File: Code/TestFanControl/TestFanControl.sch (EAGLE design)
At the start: 6 parts, among them T1 BC548

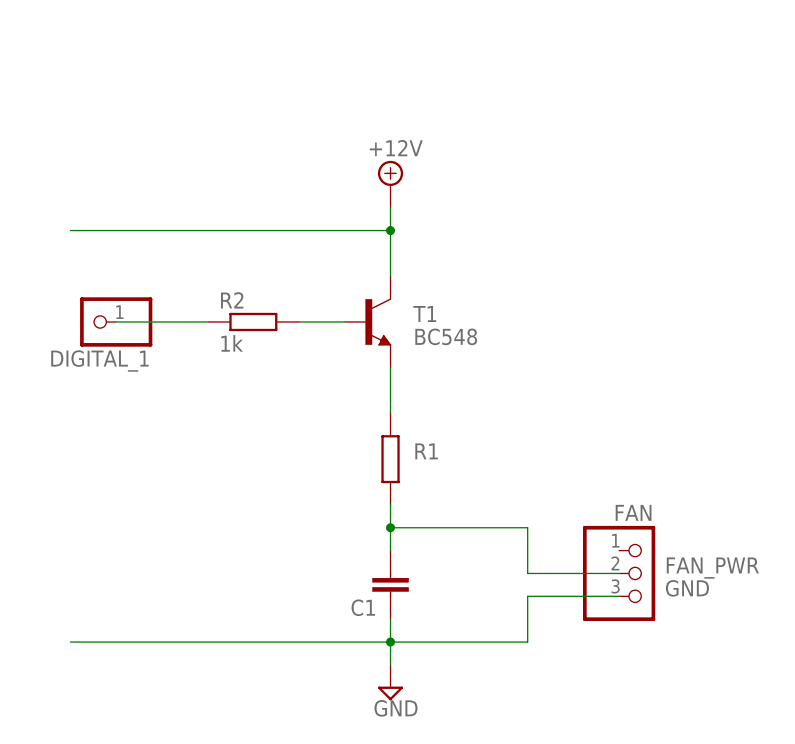
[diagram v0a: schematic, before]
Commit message: Testing
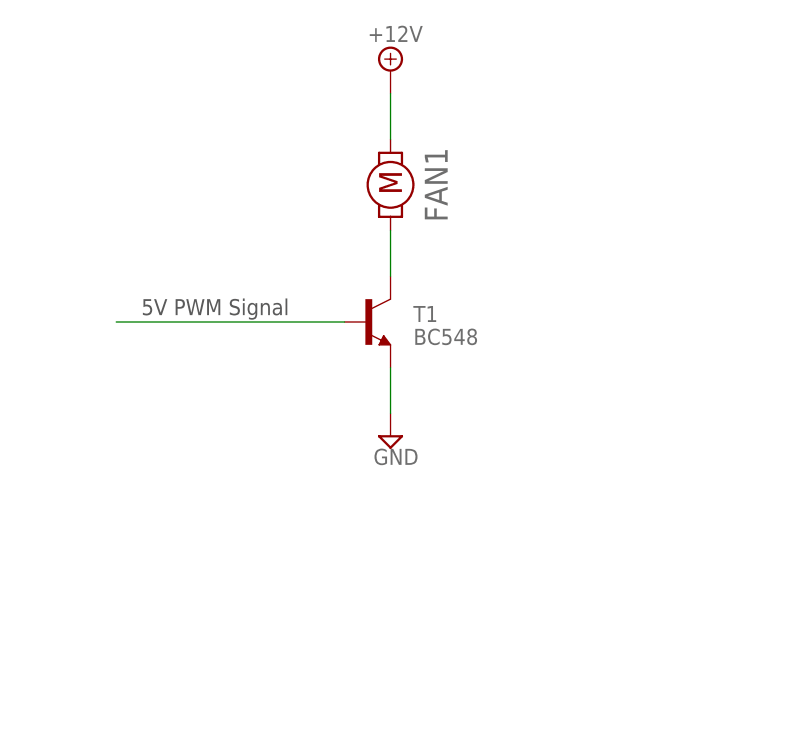
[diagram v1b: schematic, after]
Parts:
- removed C1: (no value), rcl:C-EU025-024X044
- removed DIGITAL_1: (no value), pinhead:PINHD-1X1
- removed FAN: (no value), pinhead:PINHD-1X3
- removed R1: (no value), rcl:R-EU_0204/7
- removed R2: 1k, rcl:R-EU_0204/7
- added FAN1: FAN, EnigmaMon:FAN
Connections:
- removed net FAN7_PWM: DIGITAL_1.1, R2.1
- removed net FAN_PWR: C1.2, FAN.2, R1.2
- removed net N$9: R1.1, T1.E
- new net N$2: FAN1.1, T1.C
- net +12V: now also FAN1.2; no longer T1.C
- net GND: now also T1.E; no longer C1.1, FAN.3
- net N$8: no longer R2.2
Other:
- note added: "5V PWM Signal"
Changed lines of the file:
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@@
 </classes>
 <parts>
-<part name="FAN" library="pinhead" deviceset="PINHD-1X3" device=""/>
 <part name="SUPPLY13" library="EnigmaMon" deviceset="+12V" device=""/>
 <part name="SUPPLY2" library="Rodentometer" deviceset="GND" device=""/>
 <part name="T1" library="transistor" deviceset="BC547" device="" value="BC548"/>
-<part name="R2" library="rcl" deviceset="R-EU_" device="0204/7" value="1k"/>
-<part name="DIGITAL_1" library="pinhead" deviceset="PINHD-1X1" device=""/>
-<part name="R1" library="rcl" deviceset="R-EU_" device="0204/7"/>
-<part name="C1" library="rcl" deviceset="C-EU" device="025-024X044"/>
+<part name="FAN1" library="EnigmaMon" deviceset="FAN" device=""/>
 </parts>
 <sheets>
 <sheet>
 <plain>
+<text x="5.334" y="49.022" size="1.778" layer="97">5V PWM Signal</text>
 </plain>
 <instances>
-<instance part="FAN" gate="A" x="60.96" y="20.32" smashed="yes">
-<attribute name="VALUE" x="59.69" y="12.7" size="1.778" layer="96"/>
-<attribute name="NAME" x="62.23" y="26.162" size="1.778" layer="95" rot="MR0"/>
-</instance>
-<instance part="SUPPLY13" gate="+12V" x="33.02" y="63.5"/>
-<instance part="SUPPLY2" gate="GND" x="33.02" y="7.62"/>
+<instance part="SUPPLY13" gate="+12V" x="33.02" y="76.2"/>
+<instance part="SUPPLY2" gate="GND" x="33.02" y="35.56"/>
 <instance part="T1" gate="G$1" x="30.48" y="48.26" smashed="yes">
 <attribute name="NAME" x="35.56" y="48.26" size="1.778" layer="95"/>
 <attribute name="VALUE" x="35.56" y="45.72" size="1.778" layer="96"/>
 </instance>
-<instance part="R2" gate="G$1" x="17.78" y="48.26"/>
-<instance part="DIGITAL_1" gate="G$1" x="0" y="48.26" rot="R180"/>
-<instance part="R1" gate="G$1" x="33.02" y="33.02" smashed="yes" rot="R270">
-<attribute name="NAME" x="35.56" y="32.9946" size="1.778" layer="95"/>
-<attribute name="VALUE" x="35.56" y="33.02" size="1.778" layer="96"/>
-</instance>
-<instance part="C1" gate="G$1" x="33.02" y="17.78" rot="R180"/>
+<instance part="FAN1" gate="G$1" x="33.02" y="63.5" rot="R90"/>
 </instances>
 <busses>
@@
 <segment>
 <pinref part="SUPPLY13" gate="+12V" pin="+12V"/>
-<pinref part="T1" gate="G$1" pin="C"/>
-<wire x1="33.02" y1="60.96" x2="33.02" y2="58.42" width="0.1524" layer="91"/>
-<wire x1="33.02" y1="58.42" x2="33.02" y2="53.34" width="0.1524" layer="91"/>
-<wire x1="33.02" y1="58.42" x2="-2.54" y2="58.42" width="0.1524" layer="91"/>
-<junction x="33.02" y="58.42"/>
-</segment>
-</net>
-<net name="GND" class="0">
-<segment>
-<wire x1="33.02" y1="15.24" x2="33.02" y2="12.7" width="0.1524" layer="91"/>
-<pinref part="SUPPLY2" gate="GND" pin="GND"/>
-<pinref part="C1" gate="G$1" pin="1"/>
-<pinref part="FAN" gate="A" pin="3"/>
-<wire x1="33.02" y1="12.7" x2="33.02" y2="10.16" width="0.1524" layer="91"/>
-<wire x1="58.42" y1="17.78" x2="48.26" y2="17.78" width="0.1524" layer="91"/>
-<wire x1="48.26" y1="17.78" x2="48.26" y2="12.7" width="0.1524" layer="91"/>
-<wire x1="48.26" y1="12.7" x2="33.02" y2="12.7" width="0.1524" layer="91"/>
-<label x="63.5" y="17.78" size="1.778" layer="95"/>
-<junction x="33.02" y="12.7"/>
-<wire x1="33.02" y1="12.7" x2="-2.54" y2="12.7" width="0.1524" layer="91"/>
+<wire x1="33.02" y1="68.58" x2="33.02" y2="73.66" width="0.1524" layer="91"/>
+<pinref part="FAN1" gate="G$1" pin="2"/>
 </segment>
 </net>
@@
 <segment>
 <pinref part="T1" gate="G$1" pin="B"/>
-<wire x1="27.94" y1="48.26" x2="22.86" y2="48.26" width="0.1524" layer="91"/>
-<pinref part="R2" gate="G$1" pin="2"/>
+<wire x1="27.94" y1="48.26" x2="2.54" y2="48.26" width="0.1524" layer="91"/>
 </segment>
 </net>
-<net name="FAN7_PWM" class="0">
+<net name="N$2" class="0">
 <segment>
-<pinref part="R2" gate="G$1" pin="1"/>
-<wire x1="12.7" y1="48.26" x2="2.54" y2="48.26" width="0.1524" layer="91"/>
-<pinref part="DIGITAL_1" gate="G$1" pin="1"/>
+<pinref part="T1" gate="G$1" pin="C"/>
+<wire x1="33.02" y1="53.34" x2="33.02" y2="58.42" width="0.1524" layer="91"/>
+<pinref part="FAN1" gate="G$1" pin="1"/>
 </segment>
 </net>
-<net name="N$9" class="0">
+<net name="GND" class="0">
 <segment>
 <pinref part="T1" gate="G$1" pin="E"/>
-<pinref part="R1" gate="G$1" pin="1"/>
 <wire x1="33.02" y1="43.18" x2="33.02" y2="38.1" width="0.1524" layer="91"/>
+<pinref part="SUPPLY2" gate="GND" pin="GND"/>
 </segment>
 </net>
-<net name="FAN_PWR" class="0">
-<segment>
-<pinref part="R1" gate="G$1" pin="2"/>
-<wire x1="33.02" y1="27.94" x2="33.02" y2="25.4" width="0.1524" layer="91"/>
-<wire x1="33.02" y1="25.4" x2="33.02" y2="22.86" width="0.1524" layer="91"/>
-<pinref part="C1" gate="G$1" pin="2"/>
-<pinref part="FAN" gate="A" pin="2"/>
-<wire x1="58.42" y1="20.32" x2="48.26" y2="20.32" width="0.1524" layer="91"/>
-<wire x1="48.26" y1="20.32" x2="48.26" y2="25.4" width="0.1524" layer="91"/>
-<wire x1="48.26" y1="25.4" x2="33.02" y2="25.4" width="0.1524" layer="91"/>
-<label x="63.5" y="20.32" size="1.778" layer="95"/>
-<junction x="33.02" y="25.4"/>
-</segment>
-</net>
